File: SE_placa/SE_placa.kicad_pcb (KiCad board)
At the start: 2 copper layers, 114.3 x 57.4 mm, 70 parts, among them IC1 TP4056, J1 5V, J2 Micro_SD_Card_Det_Hirose_DM3AT, J3 Conn_02x07_ESP32_IO, J4 I2C-0, J5 I2C-1, J6 Conn_02x03_LORA_IO, J7 U.FL-R-SMT(01), J8 UART, J9 Connector Bateria, Q1 BSS138, Q2 BSS138, SW1 SW_Push_Download, SW2 SW_Push_ESP_RST, U1 ESP32-WROVER, U2 RFM95W-915S2, U3 LTC3441EDEPBF

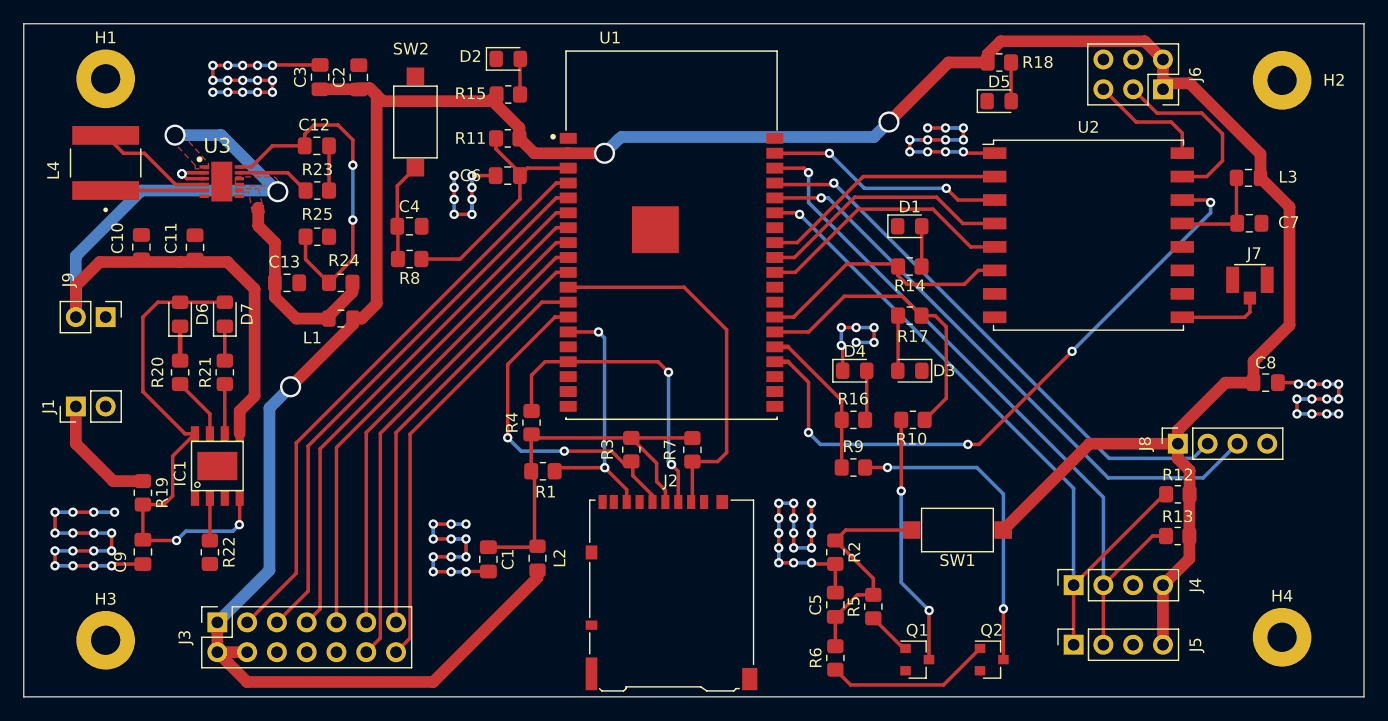
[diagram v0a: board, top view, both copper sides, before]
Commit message: Update SE_placa.kicad_pcb
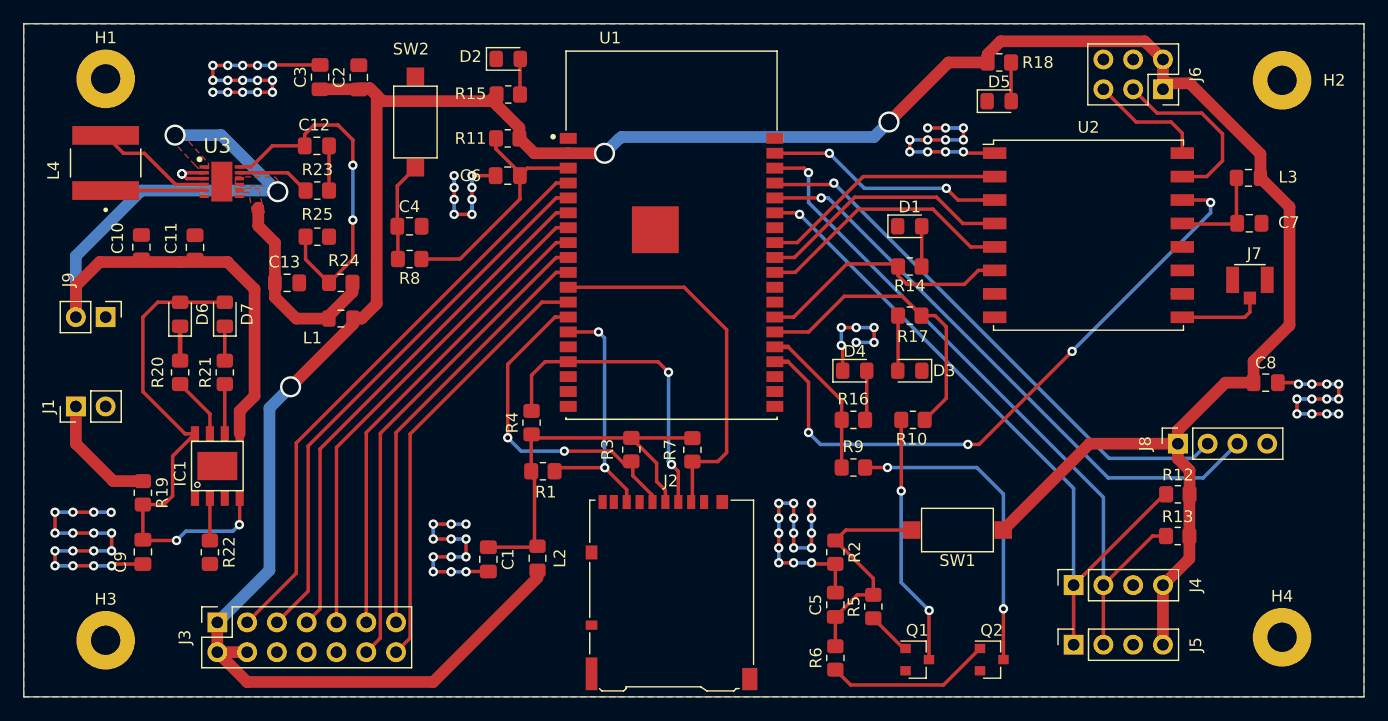
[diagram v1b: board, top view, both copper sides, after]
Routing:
- added copper zone on B.Cu, net GND
- added copper zone on F.Cu, net GND
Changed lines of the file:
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@@
     (thickness 1.6)
     (drawings 4)
-    (tracks 615)
+    (tracks 616)
     (zones 0)
     (modules 70)
@@
   (via (at 114.554 60.452) (size 0.8) (drill 0.4) (layers F.Cu B.Cu) (net 1))
   (segment (start 112.776 60.452) (end 114.554 60.452) (width 0.3) (layer F.Cu) (net 1))
-  (via (at 116.332 60.452) (size 0.8) (drill 0.4) (layers F.Cu B.Cu) (net 1))
-  (segment (start 114.554 60.452) (end 116.332 60.452) (width 0.3) (layer B.Cu) (net 1))
   (via (at 178.308 46.228) (size 0.8) (drill 0.4) (layers F.Cu B.Cu) (net 1))
   (segment (start 178.426 46.346) (end 178.308 46.228) (width 0.3) (layer F.Cu) (net 1))
@@
   (segment (start 122.4828 32.008) (end 122.0724 31.5976) (width 0.3) (layer F.Cu) (net 1))
   (segment (start 123.976 32.008) (end 122.4828 32.008) (width 0.3) (layer F.Cu) (net 1))
+  (via (at 116.0399 60.4647) (size 0.8) (drill 0.4) (layers F.Cu B.Cu) (net 1))
+  (segment (start 114.554 60.452) (end 116.0272 60.452) (width 0.3) (layer B.Cu) (net 1))
+  (segment (start 116.0272 60.452) (end 116.0399 60.4647) (width 0.3) (layer B.Cu) (net 1))
   (segment (start 151.8605 53.8475) (end 151.892 53.816) (width 0.4) (layer F.Cu) (net 2))
   (segment (start 151.8605 56.9595) (end 151.8605 53.8475) (width 0.3) (layer F.Cu) (net 2))
@@
   )
   (zone (net 50) (net_name /cargador_regulador/BAT+) (layer F.Cu) (hatch edge 0.508)
+    (priority 1)
     (connect_pads yes (clearance 0.2))
     (min_thickness 0.2)
@@
   )
   (zone (net 73) (net_name /cargador_regulador/Vout3.3V) (layer F.Cu) (hatch edge 0.508)
+    (priority 1)
     (connect_pads yes (clearance 0.2))
     (min_thickness 0.2)
@@
   )
   (zone (net 50) (net_name /cargador_regulador/BAT+) (layer F.Cu) (hatch edge 0.508)
+    (priority 1)
     (connect_pads yes (clearance 0.2))
     (min_thickness 0.2)
@@
     (polygon
       (pts
-        (xy 124.333 30.6959) (xy 124.3711 31.1531) (xy 123.2027 31.1658) (xy 123.2027 30.861) (xy 120.777 28.2575)
+        (xy 124.333 30.6959) (xy 124.3711 31.1531) (xy 123.4567 31.1277) (xy 123.2027 30.861) (xy 120.777 28.2575)
         (xy 121.5644 27.6225)
       )
     )
+  )
+  (zone (net 1) (net_name GND) (layer F.Cu) (hatch edge 0.508)
+    (connect_pads yes (clearance 0.2))
+    (min_thickness 0.2)
+    (fill yes (arc_segments 32) (thermal_gap 0.508) (thermal_bridge_width 0.508))
+    (polygon
+      (pts
+        (xy 222.885 18.796) (xy 222.885 76.2) (xy 108.585 76.1873) (xy 108.5977 18.7833)
+      )
+    )
+  )
+  (zone (net 1) (net_name GND) (layer B.Cu) (hatch edge 0.508)
+    (connect_pads yes (clearance 0.2))
+    (min_thickness 0.2)
+    (fill yes (arc_segments 32) (thermal_gap 0.508) (thermal_bridge_width 0.508))
+    (polygon
+      (pts
+        (xy 222.885 76.2) (xy 108.585 76.2) (xy 108.585 18.796) (xy 222.885 18.796)
+      )
+    )
